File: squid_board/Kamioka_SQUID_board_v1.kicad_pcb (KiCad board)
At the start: 2 copper layers, 72 x 110 mm, 18 parts, among them J1 Conn_01x25, J6 Conn_01x51

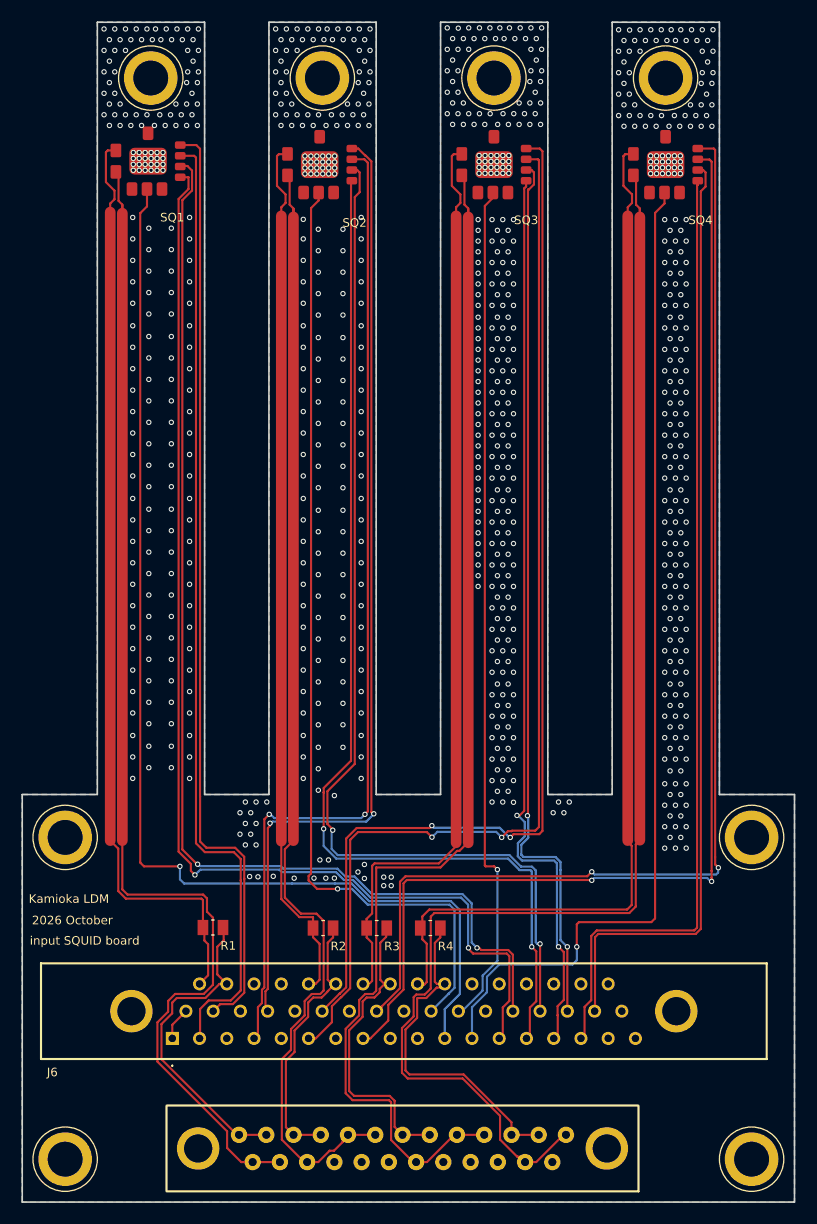
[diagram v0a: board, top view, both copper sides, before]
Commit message: latest update
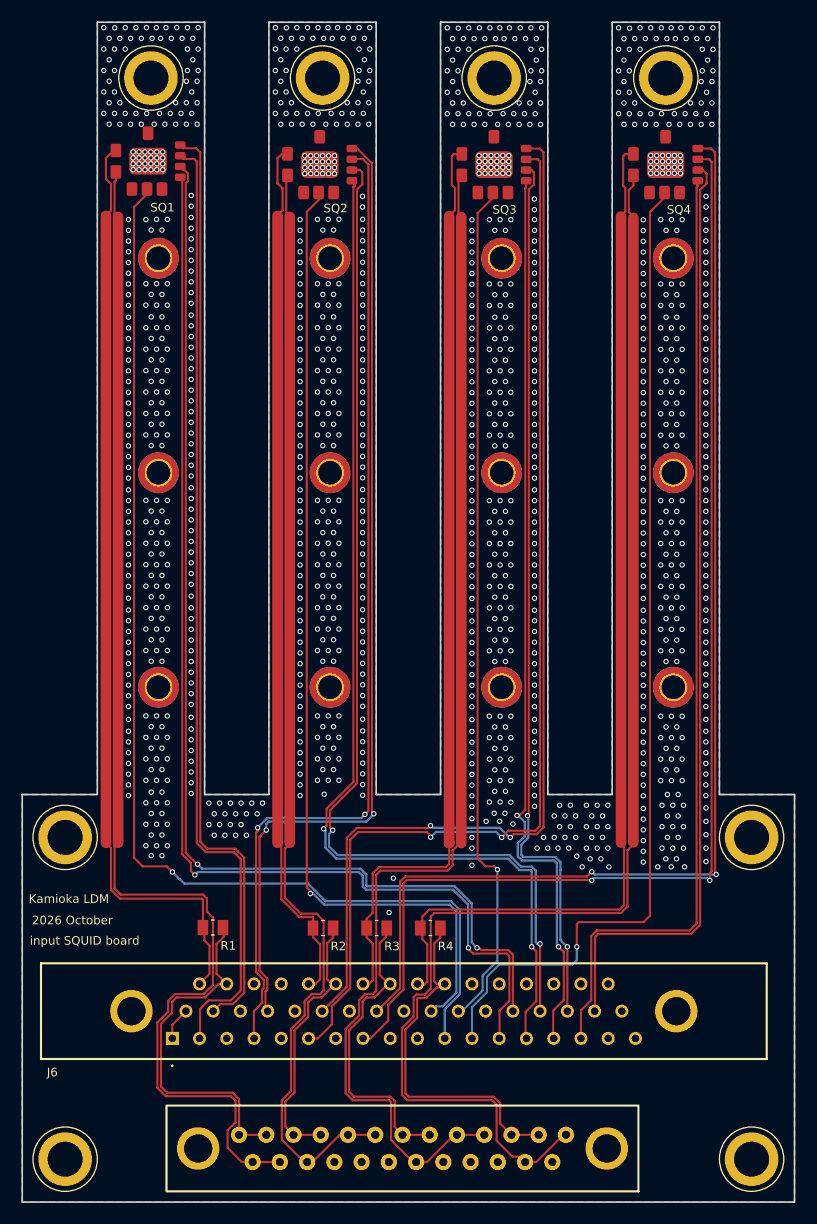
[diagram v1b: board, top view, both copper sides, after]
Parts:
- added H10: MountingHole_Pad, MountingHole:MountingHole_2.2mm_M2_DIN965_Pad_TopBottom, F.Cu at (112.7, 70.0)
- added H11: MountingHole_Pad, MountingHole:MountingHole_2.2mm_M2_DIN965_Pad_TopBottom, F.Cu at (112.7, 90.0)
- added H12: MountingHole_Pad, MountingHole:MountingHole_2.2mm_M2_DIN965_Pad_TopBottom, F.Cu at (128.7, 50.0)
- added H13: MountingHole_Pad, MountingHole:MountingHole_2.2mm_M2_DIN965_Pad_TopBottom, F.Cu at (128.7, 70.0)
- added H14: MountingHole_Pad, MountingHole:MountingHole_2.2mm_M2_DIN965_Pad_TopBottom, F.Cu at (128.7, 90.0)
- added H15: MountingHole_Pad, MountingHole:MountingHole_2.2mm_M2_DIN965_Pad_TopBottom, F.Cu at (144.7, 50.0)
- added H16: MountingHole_Pad, MountingHole:MountingHole_2.2mm_M2_DIN965_Pad_TopBottom, F.Cu at (144.7, 70.0)
- added H17: MountingHole_Pad, MountingHole:MountingHole_2.2mm_M2_DIN965_Pad_TopBottom, F.Cu at (144.7, 90.0)
- added H18: MountingHole_Pad, MountingHole:MountingHole_2.2mm_M2_DIN965_Pad_TopBottom, F.Cu at (160.7, 50.0)
- added H19: MountingHole_Pad, MountingHole:MountingHole_2.2mm_M2_DIN965_Pad_TopBottom, F.Cu at (160.7, 70.0)
- added H20: MountingHole_Pad, MountingHole:MountingHole_2.2mm_M2_DIN965_Pad_TopBottom, F.Cu at (160.7, 90.0)
- added H9: MountingHole_Pad, MountingHole:MountingHole_2.2mm_M2_DIN965_Pad_TopBottom, F.Cu at (112.7, 50.0)
- turned H1 to 90 degrees
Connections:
- J1 pad MH2: (no net) -> GND
- J6 pad MH1: (no net) -> GND
- J6 pad MH2: (no net) -> GND
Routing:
- net /Ch1_3: track 111.2 -> 115.6 mm
- net /Ch1_1: track 29.6 -> 33.2 mm
- net /Ch2_3: track 105.6 -> 103.9 mm
- net /Ch4_1: track 32.0 -> 33.7 mm
- net /fb+sq_1: track 110.2 -> 109.0 mm
- net /h+sq_4: track 94.3 -> 93.3 mm
- net /h+sq_2: track 89.6 -> 90.5 mm
- net /I-sq_2: track 90.8 -> 91.6 mm
- net /fb+sq_2: track 99.5 -> 100.2 mm
- net /Ch4_3: track 126.3 -> 125.5 mm
- net /fb-sq_1: track 107.2 -> 106.5 mm
- net /h+sq_1: track 108.0 -> 107.3 mm
- net /Ch3_1: track 29.0 -> 28.3 mm
- net /I-sq_1: track 87.6 -> 87.0 mm
- net /I+_sq1: track 89.7 -> 89.1 mm
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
